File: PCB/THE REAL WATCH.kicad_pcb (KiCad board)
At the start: 2 copper layers, 37.5 x 37.5 mm, 48 parts, among them J1 Conn_01x02_Pin, J2 Conn_01x02_Pin, J3 Conn_01x02_Pin, J4 Conn_01x13_Pin, P1 USB_C_Plug_USB2.0, Q1 BSS84, Q2 2N7002, SW1 SW_Push, SW2 SW_Push, U1 ESP32-S3-MINI-1, U10 AP2112K-1.8, U11 BNO085, U2 MAX30102, U3 BME680, U5 TP4056-42-ESOP8, U6 AP2112K-3.3, U7 MAX98357A, U8 DRV2605LDGS, U9 LC709203FQH-01TWG

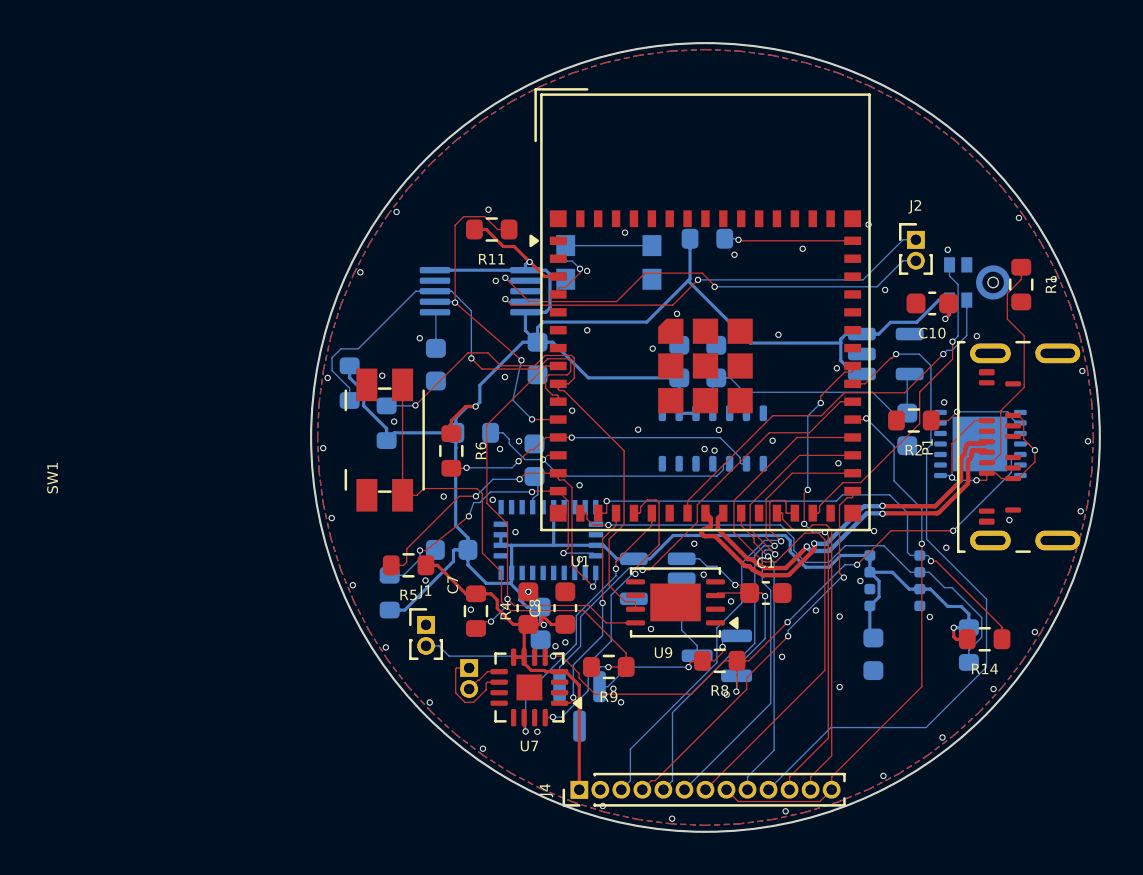
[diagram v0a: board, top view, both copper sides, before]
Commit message: Add files via upload
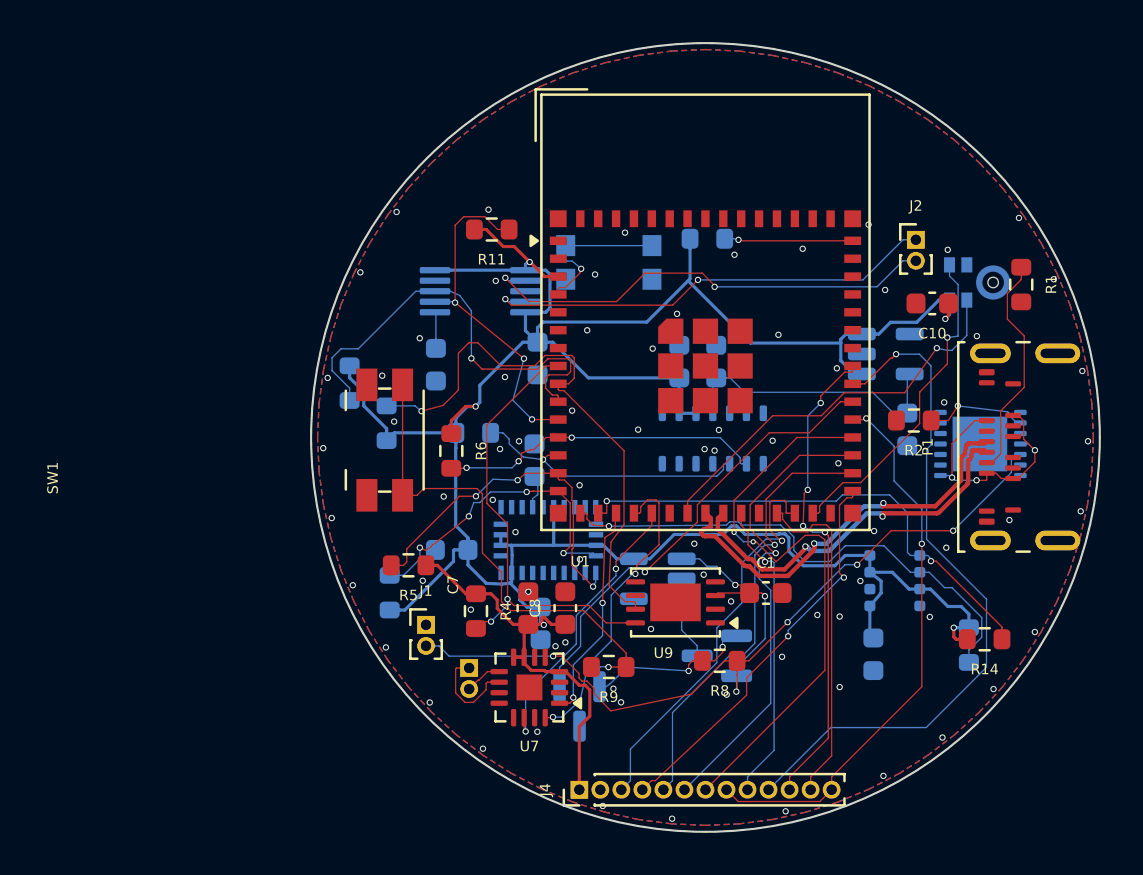
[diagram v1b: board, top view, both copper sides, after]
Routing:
- net /IO5: track 25.5 -> 27.0 mm
- net +3.3V: track 141.2 -> 142.3 mm
- net /B+: track 47.0 -> 47.6 mm
- net /IO38: track 28.0 -> 27.9 mm, vias 0 -> 2
